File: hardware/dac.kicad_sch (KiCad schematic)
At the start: 17 parts, among them J401 031-5640-1010, U401 DAC7562SDGSR, U402 MCP6001T-E/OT

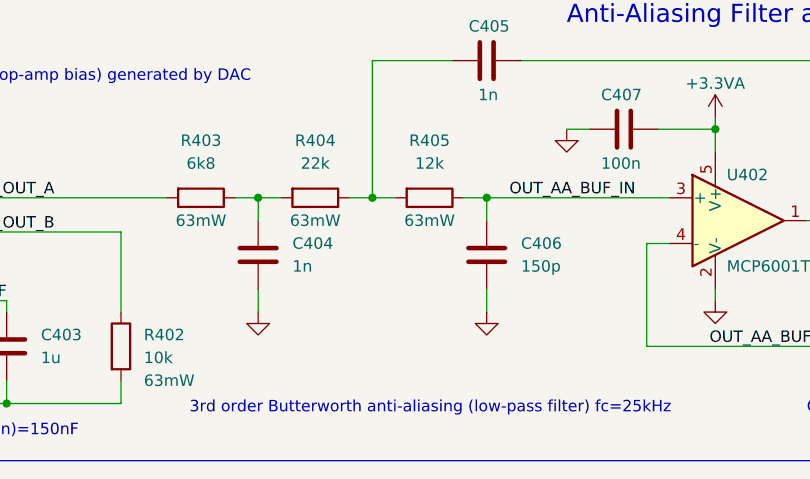
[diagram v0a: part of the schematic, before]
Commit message: Finished routing
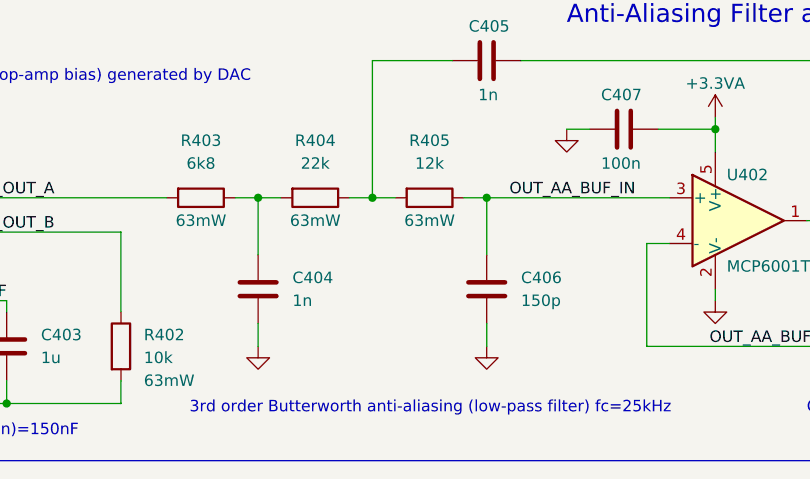
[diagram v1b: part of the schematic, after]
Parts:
- C402, C407: MPN CC0402KRX5R6BB104 -> C1525; Rating 10V -> 16V
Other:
- moved on the sheet: C404, C406
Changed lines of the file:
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@@
     (stroke (width 0) (type default))
   )
-  (wire (pts (xy 148.59 95.25) (xy 148.59 92.71))
+  (wire (pts (xy 148.59 99.06) (xy 148.59 92.71))
     (stroke (width 0) (type default))
   )
@@
     (stroke (width 0) (type default))
   )
-  (wire (pts (xy 173.99 102.87) (xy 173.99 105.41))
+  (wire (pts (xy 173.99 106.68) (xy 173.99 109.22))
     (stroke (width 0) (type default))
   )
@@
     (stroke (width 0) (type default))
   )
-  (wire (pts (xy 173.99 95.25) (xy 173.99 92.71))
+  (wire (pts (xy 173.99 99.06) (xy 173.99 92.71))
     (stroke (width 0) (type default))
   )
@@
     (stroke (width 0) (type default))
   )
-  (wire (pts (xy 148.59 102.87) (xy 148.59 105.41))
+  (wire (pts (xy 148.59 106.68) (xy 148.59 109.22))
     (stroke (width 0) (type default))
   )
@@
     )
   )
-  (symbol (lib_id "power:GND") (at 148.59 105.41 0) (unit 1)
-    (in_bom yes) (on_board yes) (dnp no)
-    (property "Reference" "#PWR0404" (at 148.59 111.76 0)
-      (effects (font (size 1.27 1.27)) hide)
-    )
-    (property "Value" "GND" (at 148.59 109.22 0)
-      (effects (font (size 1.27 1.27)) hide)
-    )
-    (property "Footprint" "" (at 148.59 105.41 0)
-      (effects (font (size 1.27 1.27)) hide)
-    )
-    (property "Datasheet" "" (at 148.59 105.41 0)
+  (symbol (lib_id "power:GND") (at 148.59 109.22 0) (unit 1)
+    (in_bom yes) (on_board yes) (dnp no)
+    (property "Reference" "#PWR0404" (at 148.59 115.57 0)
+      (effects (font (size 1.27 1.27)) hide)
+    )
+    (property "Value" "GND" (at 148.59 113.03 0)
+      (effects (font (size 1.27 1.27)) hide)
+    )
+    (property "Footprint" "" (at 148.59 109.22 0)
+      (effects (font (size 1.27 1.27)) hide)
+    )
+    (property "Datasheet" "" (at 148.59 109.22 0)
       (effects (font (size 1.27 1.27)) hide)
     )
@@
       (effects (font (size 1.27 1.27)) hide)
     )
-    (property "MPN" "CC0402KRX5R6BB104" (at 189.23 85.09 0)
-      (effects (font (size 1.27 1.27)) hide)
-    )
-    (property "Rating" "10V" (at 189.23 85.09 0)
+    (property "MPN" "C1525" (at 189.23 85.09 0)
+      (effects (font (size 1.27 1.27)) hide)
+    )
+    (property "Rating" "16V" (at 189.23 85.09 0)
       (effects (font (size 1.27 1.27)) hide)
     )
@@
     )
   )
-  (symbol (lib_id "Device:C") (at 173.99 99.06 0) (unit 1)
-    (in_bom yes) (on_board yes) (dnp no)
-    (property "Reference" "C406" (at 177.8 97.79 0)
-      (effects (font (size 1.27 1.27)) (justify left))
-    )
-    (property "Value" "150p" (at 177.8 100.33 0)
-      (effects (font (size 1.27 1.27)) (justify left))
-    )
-    (property "Footprint" "Capacitor_SMD:C_0402_1005Metric" (at 174.9552 102.87 0)
-      (effects (font (size 1.27 1.27)) hide)
-    )
-    (property "Datasheet" "~" (at 173.99 99.06 0)
+  (symbol (lib_id "Device:C") (at 173.99 102.87 0) (unit 1)
+    (in_bom yes) (on_board yes) (dnp no)
+    (property "Reference" "C406" (at 177.8 101.6 0)
+      (effects (font (size 1.27 1.27)) (justify left))
+    )
+    (property "Value" "150p" (at 177.8 104.14 0)
+      (effects (font (size 1.27 1.27)) (justify left))
+    )
+    (property "Footprint" "Capacitor_SMD:C_0402_1005Metric" (at 174.9552 106.68 0)
+      (effects (font (size 1.27 1.27)) hide)
+    )
+    (property "Datasheet" "~" (at 173.99 102.87 0)
       (effects (font (size 1.27 1.27)) hide)
     )
@@
     )
   )
-  (symbol (lib_id "Device:C") (at 148.59 99.06 0) (unit 1)
-    (in_bom yes) (on_board yes) (dnp no)
-    (property "Reference" "C404" (at 152.4 97.79 0)
-      (effects (font (size 1.27 1.27)) (justify left))
-    )
-    (property "Value" "1n" (at 152.4 100.33 0)
-      (effects (font (size 1.27 1.27)) (justify left))
-    )
-    (property "Footprint" "Capacitor_SMD:C_0402_1005Metric" (at 149.5552 102.87 0)
-      (effects (font (size 1.27 1.27)) hide)
-    )
-    (property "Datasheet" "~" (at 148.59 99.06 0)
+  (symbol (lib_id "Device:C") (at 148.59 102.87 0) (unit 1)
+    (in_bom yes) (on_board yes) (dnp no)
+    (property "Reference" "C404" (at 152.4 101.6 0)
+      (effects (font (size 1.27 1.27)) (justify left))
+    )
+    (property "Value" "1n" (at 152.4 104.14 0)
+      (effects (font (size 1.27 1.27)) (justify left))
+    )
+    (property "Footprint" "Capacitor_SMD:C_0402_1005Metric" (at 149.5552 106.68 0)
+      (effects (font (size 1.27 1.27)) hide)
+    )
+    (property "Datasheet" "~" (at 148.59 102.87 0)
       (effects (font (size 1.27 1.27)) hide)
     )
@@
     )
   )
-  (symbol (lib_id "power:GND") (at 173.99 105.41 0) (unit 1)
-    (in_bom yes) (on_board yes) (dnp no)
-    (property "Reference" "#PWR0405" (at 173.99 111.76 0)
-      (effects (font (size 1.27 1.27)) hide)
-    )
-    (property "Value" "GND" (at 173.99 109.22 0)
-      (effects (font (size 1.27 1.27)) hide)
-    )
-    (property "Footprint" "" (at 173.99 105.41 0)
-      (effects (font (size 1.27 1.27)) hide)
-    )
-    (property "Datasheet" "" (at 173.99 105.41 0)
+  (symbol (lib_id "power:GND") (at 173.99 109.22 0) (unit 1)
+    (in_bom yes) (on_board yes) (dnp no)
+    (property "Reference" "#PWR0405" (at 173.99 115.57 0)
+      (effects (font (size 1.27 1.27)) hide)
+    )
+    (property "Value" "GND" (at 173.99 113.03 0)
+      (effects (font (size 1.27 1.27)) hide)
+    )
+    (property "Footprint" "" (at 173.99 109.22 0)
+      (effects (font (size 1.27 1.27)) hide)
+    )
+    (property "Datasheet" "" (at 173.99 109.22 0)
       (effects (font (size 1.27 1.27)) hide)
     )
@@
       (effects (font (size 1.27 1.27)) hide)
     )
-    (property "MPN" "CC0402KRX5R6BB104" (at 82.55 77.47 0)
-      (effects (font (size 1.27 1.27)) hide)
-    )
-    (property "Rating" "10V" (at 82.55 77.47 0)
-      (effects (font (size 1.27 1.27)) hide)
-    )
+    (property "MPN" "C1525" (at 82.55 77.47 0)
+      (effects (font (size 1.27 1.27)) hide)
+    )
+    (property "Rating" "16V" (at 82.55 77.47 0)
+      (effects (font (size 1.27 1.27)) hide)
+    )
